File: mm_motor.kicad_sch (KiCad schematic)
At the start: 1 part, among them M1 N20_encoder

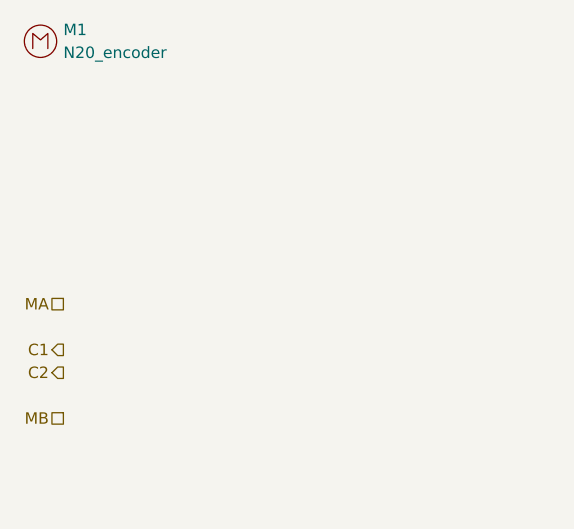
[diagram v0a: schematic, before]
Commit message: TP3
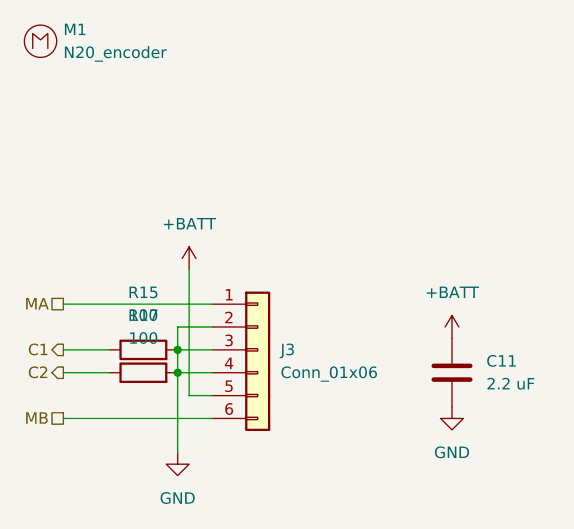
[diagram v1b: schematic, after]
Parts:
- added C11: 2.2 uF, Capacitor_SMD:C_0603_1608Metric, symbol Device:C
- added J3: Conn_01x06, Connector_PinHeader_2.54mm:PinHeader_1x06_P2.54mm_Vertical, symbol Connector_Generic:Conn_01x06
- added R15, R17: 100, Resistor_SMD:R_0603_1608Metric, symbol Device:R
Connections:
- net C1: now also R15.1
- net C2: now also R17.1
- net MA: now also J3.1 (Pin_1)
- net MB: now also J3.6 (Pin_6)
- new net +BATT: C11.1, J3.5 (Pin_5)
- new net GND: C11.2, J3.2 (Pin_2), J3.3 (Pin_3), J3.4 (Pin_4), R15.2, R17.2
